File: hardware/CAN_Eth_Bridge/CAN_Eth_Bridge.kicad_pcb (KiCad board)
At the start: 2 copper layers, 60 x 100 mm, 161 parts, among them J101 Main Current Hall Sensor, J102 Global LV and CAN, J103 HRLV, J105 Conn_02x05_Odd_Even, J106 uart, J107 Micro_SD_Card, J301 RJ45_Amphenol_RJMG1BD3B8K1ANR, K101 G5Q-1A 24Vdc, Q101 MMBT5550L, Q102 MMBT5550L, Q103 MMBT5550L, Q301 MMBT5550L, Q302 MMBT5550L, Q501 MMBT5550L, Q502 MMBT5550L, U101 MCP2542FDxMF, U102 MCP2542FDxMF, U105 XM0G3507QPTRQ1, U201 Si1450DH, U202 LM74502, U203 Si1450DH, U204 AP64060ZQ, U205 AP64060ZQ, U301 W5500, U401 MCP1501-40xSN, U402 TLV713185PDBV, U404 MCP33151, U405 MCP33151, U408 Si1450DH, U409 NCV68061, U501 NSI5030, U502 Si1450DH, U503 NCV68061, U504 MCP2542FDxMF, U505 AP7384-50SA, U506 ISOM8110, U507 ISOM8110, U508 STISO620, Y301 Crystal_GND24

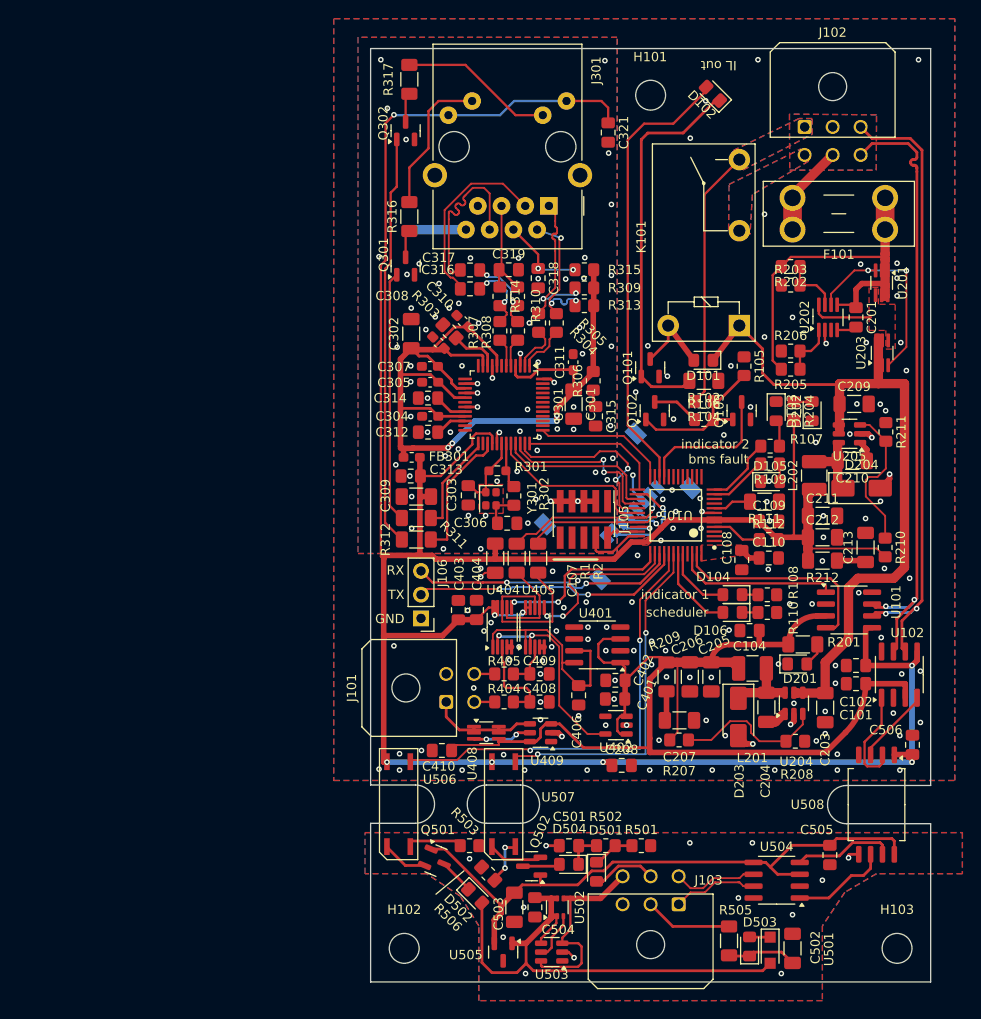
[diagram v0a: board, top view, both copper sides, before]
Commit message: long 88 can stick
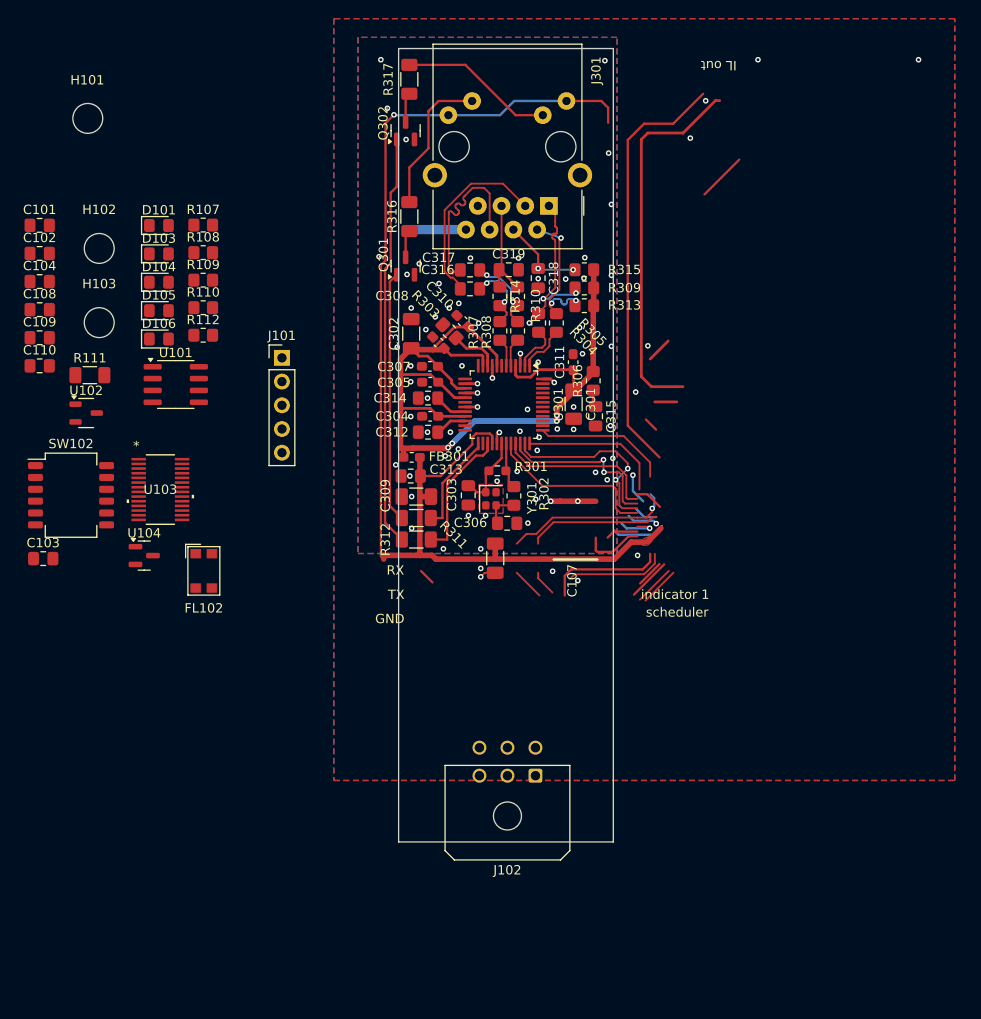
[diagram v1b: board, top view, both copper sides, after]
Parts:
- removed C201, C208, C321, C401, C402, C403, C404, C408, C409, C410, C501, C504, C505, C506: 220n, Capacitor_SMD:C_0805_2012Metric_Pad1.18x1.45mm_HandSolder
- removed C203, C205, C206, C207, C209, C211, C212, C213: 10u, Capacitor_SMD:C_1206_3216Metric_Pad1.33x1.80mm_HandSolder
- removed C204, C210: 100n, Capacitor_SMD:C_1206_3216Metric_Pad1.33x1.80mm_HandSolder
- removed C406: 10n, Capacitor_SMD:C_0805_2012Metric_Pad1.18x1.45mm_HandSolder
- removed C502, C503: 1u, Capacitor_SMD:C_1206_3216Metric_Pad1.33x1.80mm_HandSolder
- removed D102, D201, D202: green, LED_SMD:LED_0805_2012Metric_Pad1.15x1.40mm_HandSolder
- removed D203, D204: ES1D, Diode_SMD:D_SMA
- removed D501, D502, D503: TS4148, Diode_SMD:D_0805_2012Metric_Pad1.15x1.40mm_HandSolder
- removed D504: 10V, Diode_SMD:D_0805_2012Metric_Pad1.15x1.40mm_HandSolder
- removed F101: ~1A, Fuse:Fuseholder_Blade_Mini_Keystone_3568
- removed J103: HRLV, Connector_Molex:Molex_Micro-Fit_3.0_43045-0600_2x03_P3.00mm_Horizontal
- removed J105: Conn_02x05_Odd_Even, Connector_PinHeader_1.27mm:PinHeader_2x05_P1.27mm_Vertical_SMD
- removed J106: uart, Connector_PinHeader_2.54mm:PinHeader_1x03_P2.54mm_Vertical
- removed J107: Micro_SD_Card, Connector_Card:microSD_HC_Wuerth_693072010801
- removed K101: G5Q-1A 24Vdc, Relay_THT:Relay_SPST_Omron-G5Q-1A
- removed L201, L202: 10u, Inductor_SMD:L_1210_3225Metric_Pad1.42x2.65mm_HandSolder
- removed Q101, Q102, Q103, Q501, Q502: MMBT5550L, Package_TO_SOT_SMD:SOT-23
- removed R1, R2, R505: 100, Resistor_SMD:R_1206_3216Metric_Pad1.30x1.75mm_HandSolder
- removed R102, R201: 4.99k, Resistor_SMD:R_1206_3216Metric_Pad1.30x1.75mm_HandSolder
- removed R104, R202, R501: 88.7k, Resistor_SMD:R_0805_2012Metric_Pad1.20x1.40mm_HandSolder
- removed R105, R203, R204: 3.32k, Resistor_SMD:R_0805_2012Metric_Pad1.20x1.40mm_HandSolder
- removed R106: 49.9, Resistor_SMD:R_0805_2012Metric_Pad1.20x1.40mm_HandSolder
- removed R205: 140k, Resistor_SMD:R_0805_2012Metric_Pad1.20x1.40mm_HandSolder
- removed R206, R208, R211: 22.1k, Resistor_SMD:R_0805_2012Metric_Pad1.20x1.40mm_HandSolder
- removed R207: 88.7kR, Resistor_SMD:R_0805_2012Metric_Pad1.20x1.40mm_HandSolder
- removed R209, R212: 4.7, Resistor_SMD:R_1206_3216Metric_Pad1.30x1.75mm_HandSolder
- removed R210: 51k, Resistor_SMD:R_0805_2012Metric_Pad1.20x1.40mm_HandSolder
- removed R404, R405: 14.3, Resistor_SMD:R_0805_2012Metric_Pad1.20x1.40mm_HandSolder
- removed R502, R503, R506: 2.4k, Resistor_SMD:R_0805_2012Metric_Pad1.20x1.40mm_HandSolder
- removed U105: XM0G3507QPTRQ1, zzLocalLibraries-Footprints:PT0048A-IPC_B
- removed U201, U203, U408: Si1450DH, Package_TO_SOT_SMD:SOT-363_SC-70-6_Handsoldering
- removed U202: LM74502, Package_TO_SOT_SMD:SOT-23-8_Handsoldering
- removed U204, U205: AP64060ZQ, Package_TO_SOT_SMD:TSOT-23-6
- removed U401: MCP1501-40xSN, Package_SO:SOIC-8_3.9x4.9mm_P1.27mm
- removed U402: TLV713185PDBV, Package_TO_SOT_SMD:SOT-23-5
- removed U404, U405: MCP33151, Package_SO:MSOP-10_3x3mm_P0.5mm
- removed U409, U503: NCV68061, Package_TO_SOT_SMD:TSOT-23-6
- removed U501: NSI5030, Diode_SMD:Nexperia_CFP3_SOD-123W
- removed U502: Si1450DH, Package_TO_SOT_SMD:SOT-363_SC-70-6
- removed U504: MCP2542FDxMF, Package_SO:SOIC-8_3.9x4.9mm_P1.27mm
- removed U505: AP7384-50SA, Package_TO_SOT_SMD:SOT-23
- removed U506, U507: ISOM8110, zzLocalLibraries-Footprints:ISOM811_SOIC-4_DFG
- removed U508: STISO620, Package_SO:SOIC-8_7.5x5.85mm_P1.27mm
- added C103: 220n, Capacitor_SMD:C_0805_2012Metric_Pad1.18x1.45mm_HandSolder, F.Cu at (94.9, 114.6)
- added FL102: Choke_CommonMode_FerriteCore_1243, Inductor_SMD:L_CommonModeChoke_Coilcraft_1812CAN, F.Cu at (112.1, 116.0)
- added SW102: SW_DIP_x06, Button_Switch_SMD:SW_DIP_SPSTx06_Slide_Copal_CHS-06B_W7.62mm_P1.27mm, F.Cu at (97.9, 107.9)
- added U103: XMSM0G3507SDGS28R, zzLocalLibraries-Footprints:VSSOP28_DGS_TEX-M, F.Cu at (107.5, 107.2)
- added U104: AP7381-33SA-7, Package_TO_SOT_SMD:SOT-23, F.Cu at (105.7, 114.3)
- J101: value Main Current Hall Sensor -> Conn_01x05_Pin; footprint Connector_Molex:Molex_Micro-Fit_3.0_43045-0400_2x02_P3.00mm_Horizontal -> Connector_PinHeader_2.54mm:PinHeader_1x05_P2.54mm_Vertical
- U102: value MCP2542FDxMF -> AP7384-50SA; footprint Package_SO:SOIC-8_3.9x4.9mm_P1.27mm -> Package_TO_SOT_SMD:SOT-23-3
- moved H103 108.6 mm to (100.9, 89.4)
- moved C101 100.3 mm to (94.5, 78.9), turned to 0 degrees
- moved C102 98.0 mm to (94.5, 82.0), turned to 0 degrees
- moved U102 91.5 mm to (99.5, 99.0), turned to 0 degrees
- moved C104 84.7 mm to (94.5, 85.0), turned to 0 degrees
- moved H102 81.8 mm to (100.9, 81.4)
- moved C110 80.8 mm to (94.5, 94.0)
- moved C109 80.6 mm to (94.5, 91.0)
- moved C108 79.9 mm to (94.5, 88.0), turned to 0 degrees
- moved U101 76.1 mm to (109.1, 96.0)
- moved J102 75.2 mm to (147.7, 137.9), turned to 180 degrees
- moved R111 73.5 mm to (99.9, 95.0), turned to 0 degrees
- moved R108 70.7 mm to (112.1, 81.9)
- moved D104 70.0 mm to (107.3, 85.0), turned to 0 degrees
- moved R110 68.7 mm to (112.1, 87.8), turned to 0 degrees
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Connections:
- C101 pad 1: +5V -> +3.3V
- C102 pad 1: +3.3V -> +5V
- D101 pad 1: LV+ -> Net-(D101-K)
- D101 pad 2: Net-(D101-A) -> /GLV+
- J101 pad 1: /MCHall_5Vin -> GND
- J101 pad 2: GND -> /prog.uart_ui_rx
- J101 pad 3: /MCHall_imprecise -> /prog.uart_ui_tx
- J101 pad 4: /MCHall_percise -> /prog.SWDIO
- J102 pad 4: /G_IL- -> /G_IL+
- U101 pad 6: /G_CAN- -> Net-(U101-CANL)
- U101 pad 7: /G_CAN+ -> Net-(U101-CANH)
- U102 pad 1: /HRLV interface/CAN_RX -> Net-(D101-K)
- U102 pad 2: GND -> +5V
- U102 pad 3: +5V -> GND
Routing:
- net (no net): track 0.00 -> 186.6 mm, vias 0 -> 2
- net +3.3V: track 304.3 -> 132.7 mm, vias 9 -> 2
- net +5V: track 124.4 -> 0.00 mm
- net LV+: track 80.2 -> 0.00 mm
- net /G_CAN+: track 67.4 -> 0.00 mm, vias 2 -> 0
- net /G_CAN-: track 67.4 -> 0.00 mm, vias 2 -> 0
- net /HRLV interface/+5V: track 66.0 -> 0.00 mm
- net /HRLV interface/LV+: track 54.7 -> 0.00 mm
- net /hrlv.pres_hrlv: track 48.2 -> 0.00 mm, vias 2 -> 0
- net /IL.forward: track 47.6 -> 0.00 mm
- net Net-(D102-K): track 41.4 -> 0.00 mm
- net /GLV PSU/GLV+: track 41.2 -> 0.00 mm
- net /hrlv.pres_interlock: track 37.3 -> 0.00 mm, vias 2 -> 0
- net /prog.uart_ui_rx: track 29.2 -> 4.57 mm, vias 2 -> 0
- net /Main Current Hall Sensing/4.096Vref: track 23.9 -> 0.00 mm
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- removed copper zone on F.Cu, net /GLV PSU/passing
- removed copper zone on B.Cu, net /G_IL+
- removed copper zone on F.Cu, net /G_IL+
- removed copper zone on B.Cu, net /G_IL-
- removed copper zone on F.Cu, net /G_IL-
- removed copper zone on B.Cu, net /HRLV_LV-
- removed copper zone on F.Cu, net /HRLV_LV-
- removed copper zone on F.Cu, net /vcore
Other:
- board size 60 x 100 mm -> 23 x 85 mm
- board text removed: "600Vdc galv ISO"
- board text removed: "CAN+"
- board text removed: "CAN-"
- board text removed: "GLV+ (9,34)V"
- board text removed: "GLV-"
- board text removed: "HRLV interface"
- board text removed: "IL return"
- board text removed: "IL_B"
- board text removed: "LV+ (5.5 , 35)V"
- board text removed: "LV-"
- board text removed: "bms fault"
- board text removed: "fuse ~800mA"
- board text removed: "ground loop from LV bulk to diode crosses sense line"
- board text removed: "indicator 2"
